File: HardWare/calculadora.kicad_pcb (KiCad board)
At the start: 2 copper layers, 100 x 150 mm, 69 parts, among them J1 Screw_Terminal_01x02, J5 Conector ShiftRegister, Q1 Q_NPN_CBE, Q2 Q_Photo_NPN, SW1 chave_tactil, SW10 chave_tactil, SW11 chave_tactil, SW12 chave_tactil, SW13 chave_tactil, SW14 chave_tactil, SW15 chave_tactil, SW16 chave_tactil, SW17 chave_tactil, SW18 chave_tactil, SW19 chave_tactil, SW2 chave_tactil, SW20 chave_tactil, SW21 chave_tactil, SW22 chave_tactil, SW23 chave_tactil, SW24 chave_tactil, SW25 chave_tactil, SW26 chave_tactil, SW27 chave_tactil, SW28 chave_tactil, SW29 chave_tactil, SW3 chave_tactil, SW30 chave_tactil, SW31 chave_tactil, SW32 chave_tactil, SW4 chave_tactil, SW5 chave_tactil, SW6 chave_tactil, SW7 chave_tactil, SW8 chave_tactil, SW9 chave_tactil, U1 ESP32-DEVKIT-V1, U2 LM358, U3 LM7805_TO220, U4 M74HC595B1, U5 LCD_GRAFICO_ST920

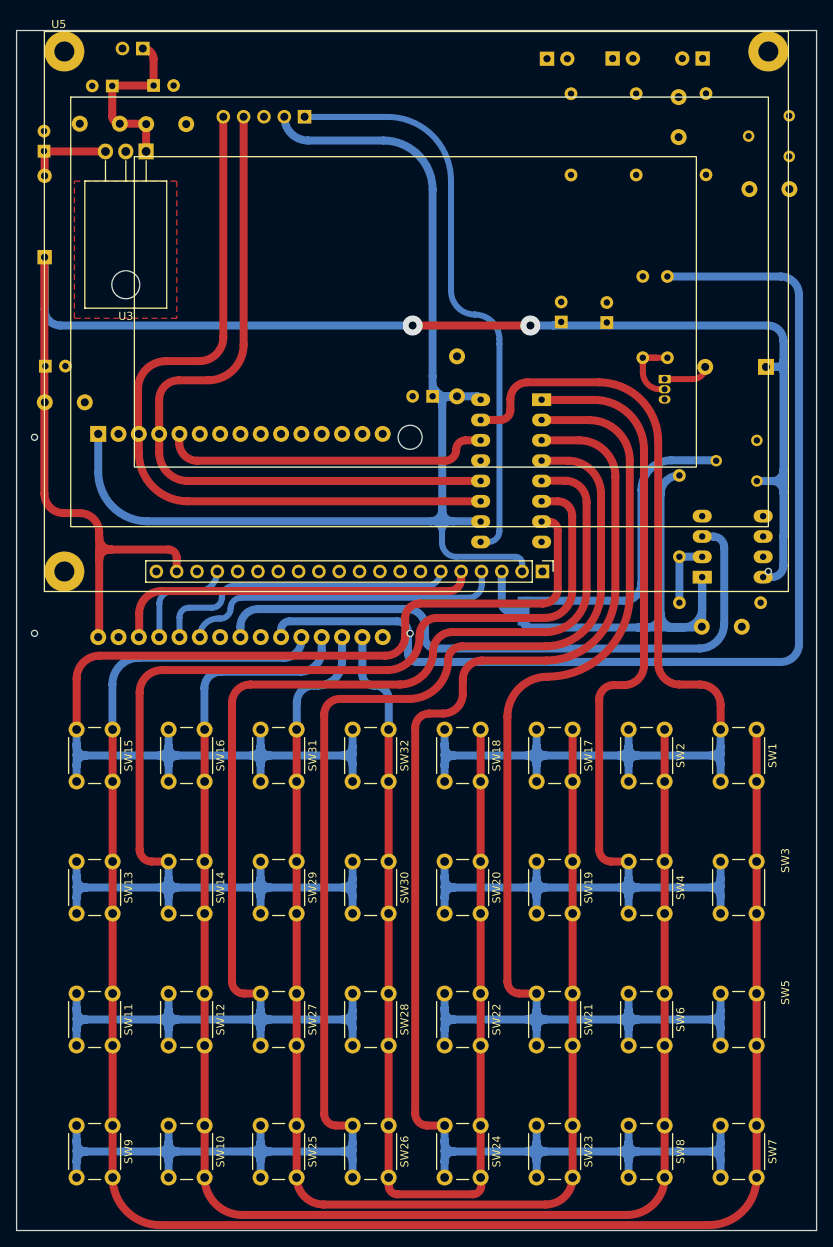
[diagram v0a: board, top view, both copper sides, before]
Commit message: Ajustes
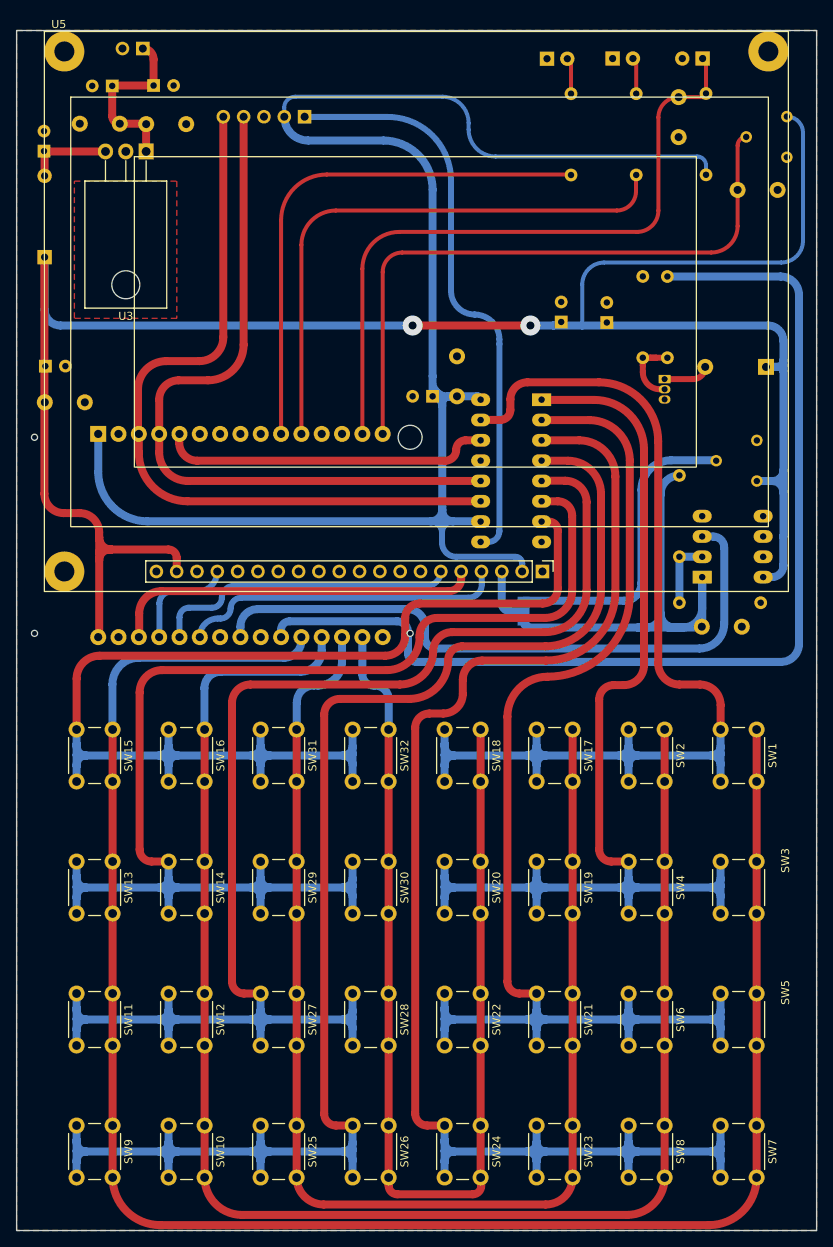
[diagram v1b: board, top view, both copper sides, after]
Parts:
- moved C3 1.48 mm to (131.1, 51.9)
- moved RV2 0.32 mm to (132.2, 47.8)
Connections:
- C18 pad 2: GNDD -> GND
- C19 pad 1: GNDD -> GND
- C2 pad 1: GNDD -> GND
- C20 pad 2: GNDD -> GND
- C23 pad 2: GNDD -> GND
- C3 pad 1: GNDD -> GND
- D2 pad 1: GNDD -> GND
- D3 pad 1: GNDD -> GND
- J5 pad 3: GNDD -> GND
- Q1 pad 3: GNDD -> GND
- Q2 pad 2: GNDD -> GND
- R4 pad 1: GNDD -> GND
- RV1 pad 3: GNDD -> GND
- RV2 pad 1: GNDD -> GND
- U1 pad 2: GNDD -> GND
- U1 pad 29: GNDD -> GND
- U4 pad 13: GNDD -> GND
- U4 pad 8: GNDD -> GND
- U5 pad 1: GNDD -> GND
- U5 pad 20: GNDD -> GND
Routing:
- net Sensor_Ir: track 0.00 -> 85.3 mm
- net Sinal_Analogico: track 0.00 -> 79.4 mm
- net Led_Red: track 0.00 -> 71.1 mm
- net Led_Ir: track 0.00 -> 66.0 mm
- net +3V3: track 157.4 -> 218.1 mm
- net +5V: track 215.6 -> 267.8 mm
- net Net-(D3-Pad2): track 0.00 -> 4.62 mm
- net Net-(D2-Pad2): track 0.00 -> 4.61 mm
- added copper zone on B.Cu, net GND
